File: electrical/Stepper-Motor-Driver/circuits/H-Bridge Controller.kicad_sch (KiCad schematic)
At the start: 0 parts

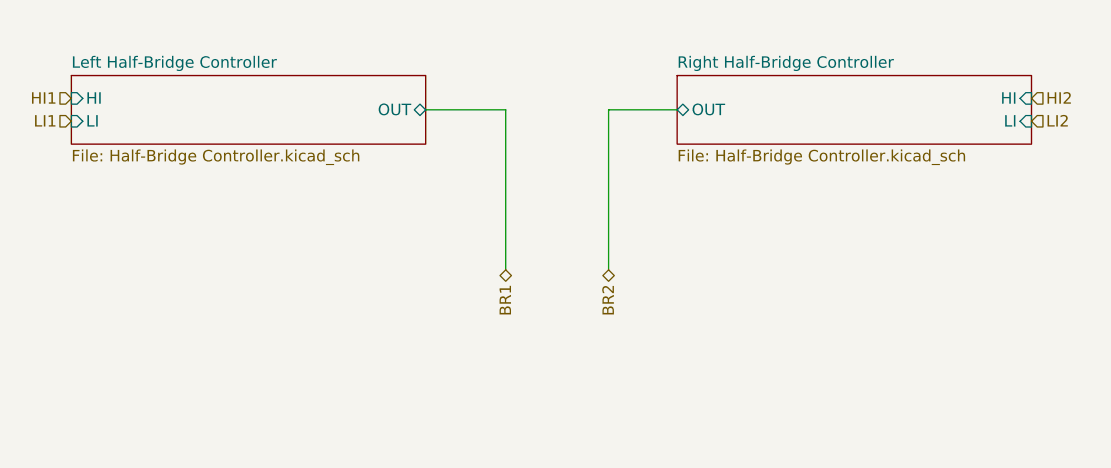
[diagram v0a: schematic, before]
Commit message: Initial PCB layout
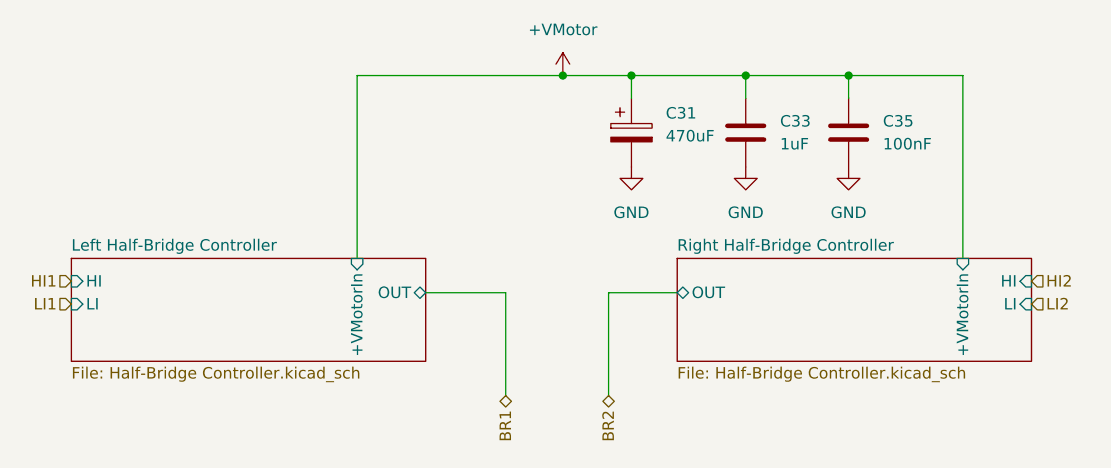
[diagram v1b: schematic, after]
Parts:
- added C31: 470uF, Capacitor_THT:CP_Radial_D12.5mm_P5.00mm, symbol Device:C_Polarized
- added C33: 1uF, Capacitor_SMD:C_1206_3216Metric, symbol Device:C
- added C35: 100nF, Capacitor_SMD:C_1206_3216Metric, symbol Device:C
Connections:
- new net +VMotor: C31.1, C33.1, C35.1
- new net GND: C31.2, C33.2, C35.2
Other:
- sheet Left Half-Bridge Controller ports: added +VMotorIn; removed none
- sheet Right Half-Bridge Controller ports: added +VMotorIn; removed none
